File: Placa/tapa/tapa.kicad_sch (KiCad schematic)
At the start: 8 parts, among them J1 Tapa, J2 Conn_01x04, SW1 Enter, SW2 ESC, SW3 Botón Selección, SW4 LR, SW5 MICRO, SW6 EMERGENCIA

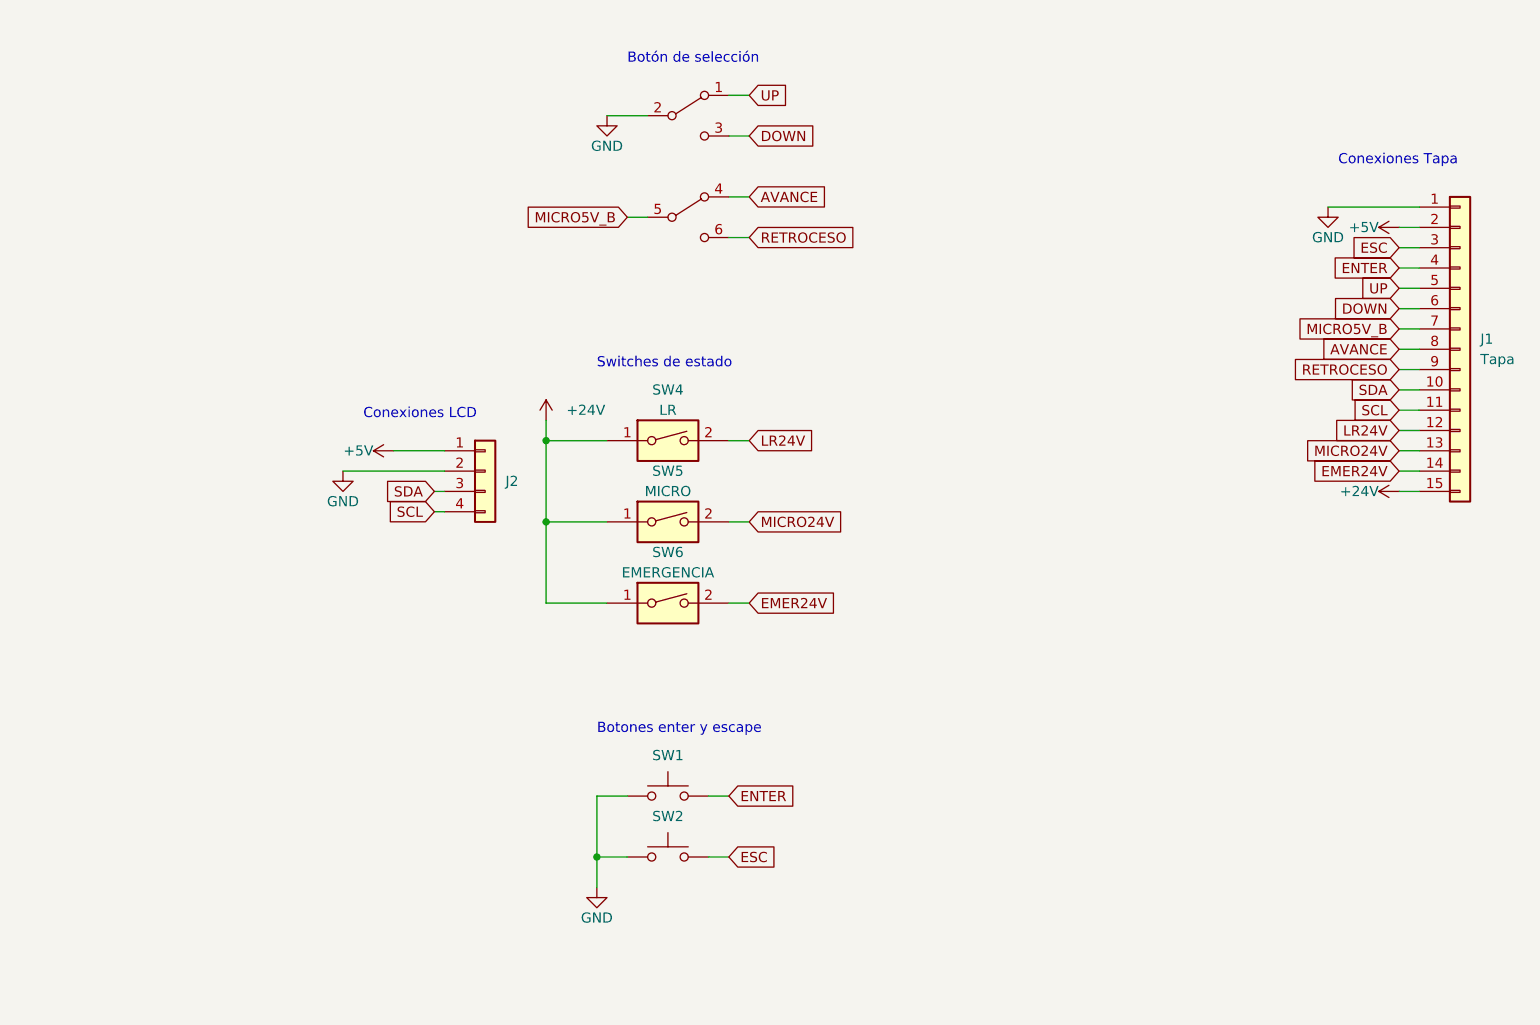
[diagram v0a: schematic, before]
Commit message: Diseño de placa
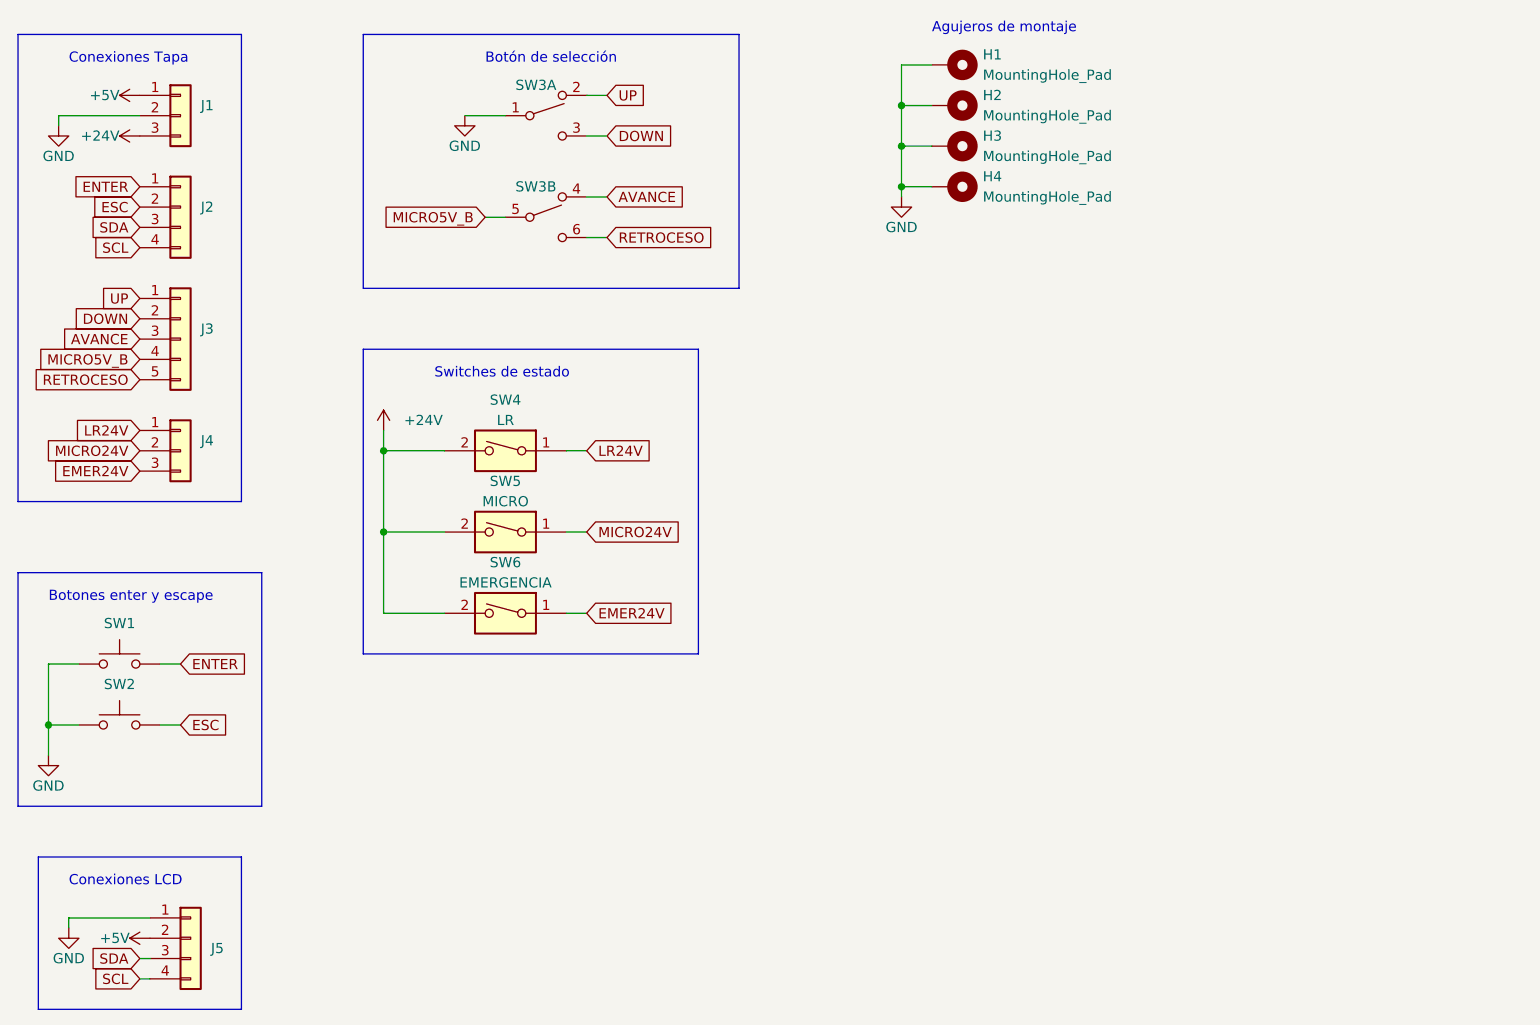
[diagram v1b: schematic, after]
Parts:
- removed J1: Tapa, symbol Connector_Generic:Conn_01x15
- added H1, H2, H3, H4: MountingHole_Pad, MountingHole:MountingHole_3.2mm_M3_DIN965_Pad, symbol Mechanical:MountingHole_Pad
- added J1, J4: Conn_01x03, TerminalBlock_TE-Connectivity:TerminalBlock_TE_282834-3_1x03_P2.54mm_Horizontal, symbol Connector_Generic:Conn_01x03
- added J2: Conn_01x04, TerminalBlock_TE-Connectivity:TerminalBlock_TE_282834-4_1x04_P2.54mm_Horizontal, symbol Connector_Generic:Conn_01x04
- added J3: Conn_01x05, TerminalBlock_TE-Connectivity:TerminalBlock_TE_282834-5_1x05_P2.54mm_Horizontal, symbol Connector_Generic:Conn_01x05
- SW3: footprint (none) -> TerminalBlock_TE-Connectivity:TerminalBlock_TE_282834-6_1x06_P2.54mm_Horizontal
- renumbered J2 to J5
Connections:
- net +24V: now also SW4.2, SW5.2, SW6.2, J1.3 (Pin_3); no longer SW4.1, SW5.1, SW6.1
- net +5V: now also J5.2 (Pin_2), J1.1 (Pin_1); no longer J5.1 (Pin_1)
- net AVANCE: now also J3.3 (Pin_3)
- net DOWN: now also J3.2 (Pin_2)
- net EMER24V: now also SW6.1, J4.3 (Pin_3); no longer SW6.2
- net ENTER: now also J2.1 (Pin_1)
- net ESC: now also J2.2 (Pin_2)
- net GND: now also J5.1 (Pin_1), SW3.1 (B), H1.1, H2.1, H3.1, H4.1, J1.2 (Pin_2); no longer J5.2 (Pin_2), SW3.2 (B)
- net LR24V: now also SW4.1, J4.1 (Pin_1); no longer SW4.2
- net MICRO24V: now also SW5.1, J4.2 (Pin_2); no longer SW5.2
- net MICRO5V_B: now also J3.4 (Pin_4)
- net RETROCESO: now also J3.5 (Pin_5)
- net SCL: now also J2.4 (Pin_4)
- net SDA: now also J2.3 (Pin_3)
- net UP: now also SW3.2 (A), J3.1 (Pin_1); no longer SW3.1 (A)
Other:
- note added: "Agujeros de montaje"
- moved on the sheet: J5, SW1, SW2, SW4, SW5, SW6
